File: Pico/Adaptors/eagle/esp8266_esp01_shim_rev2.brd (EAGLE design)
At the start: 15.9 x 11.9 mm, 4 parts, among them IC2 78L 3.3v

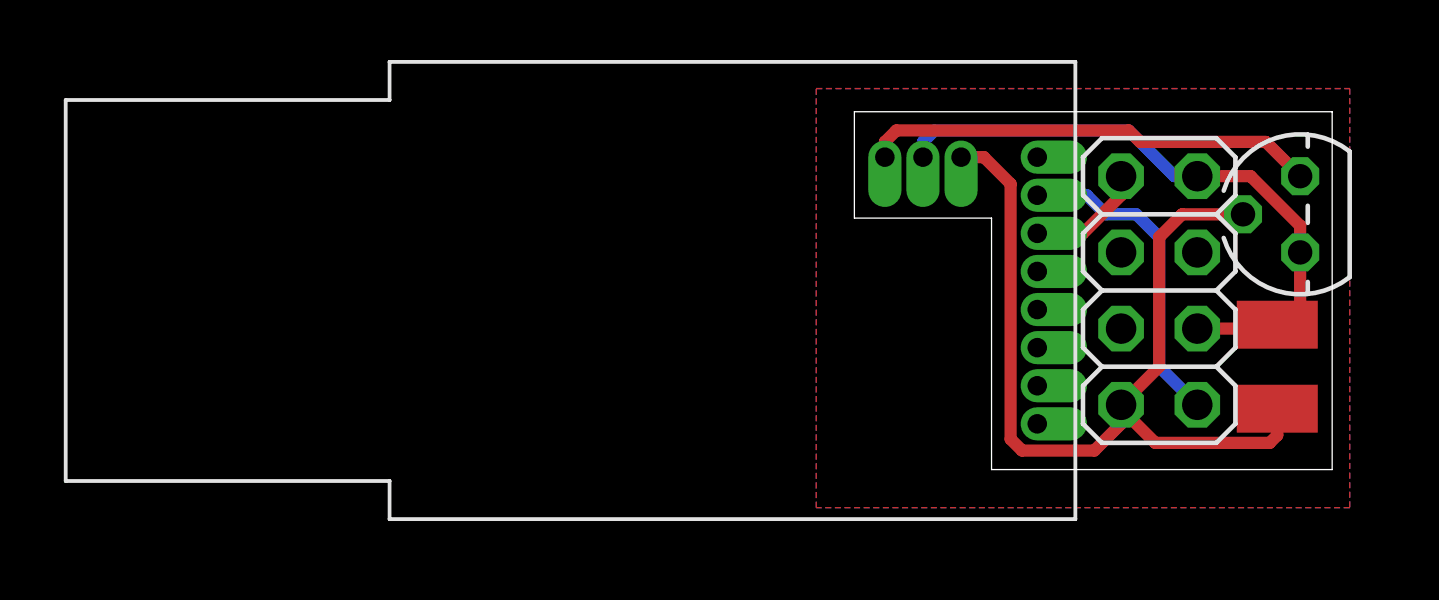
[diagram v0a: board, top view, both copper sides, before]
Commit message: tweak net classes
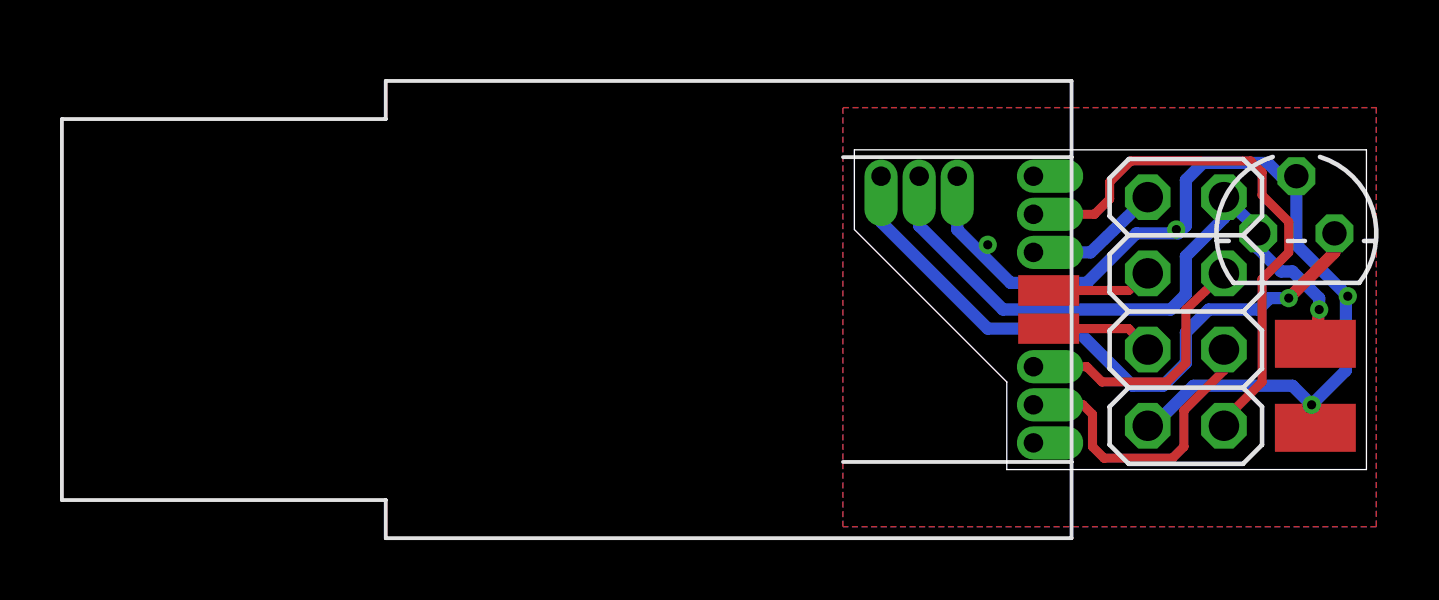
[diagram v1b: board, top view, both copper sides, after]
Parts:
- U$1: value ESPRUINO_PICO_0.05 -> ESPRUINO_PICO_0.05_SMALL; device espruino_pico:ESPRUINO_PICO_0.05 -> espruino_pico:ESPRUINO_PICO_0.05_SMALL
- moved C1 1.42 mm to (15.4, 2.79)
- moved U$1 1.31 mm to (0.89, 5.33)
- moved ESP8266 1.13 mm to (11.0, 5.27)
- moved IC2 0.65 mm to (14.7, 7.87), turned to 0 degrees
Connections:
- new net ESP_CH_PD: ESP8266.6, U$1.B9
- new net ESP_GPIO0: ESP8266.3, U$1.A1
- new net ESP_GPIO2: ESP8266.5, U$1.A0
- new net ESP_RST: ESP8266.4, U$1.A10
- net VCC: no longer ESP8266.6
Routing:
- net ESP_CH_PD: track 0.00 -> 10.3 mm
- net ESP_RST: track 0.00 -> 9.08 mm
- net ESP_TX: track 10.8 -> 18.6 mm
- net N$1: track 15.1 -> 22.0 mm, vias 0 -> 1
- net ESP_GPIO2: track 0.00 -> 3.61 mm
- net ESP_GPIO0: track 0.00 -> 3.52 mm
- net VCC: track 21.0 -> 22.6 mm, vias 0 -> 1
- net GND: track 31.4 -> 32.4 mm, vias 0 -> 4
- net ESP_RX: track 3.96 -> 4.55 mm
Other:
- board size 15.9 x 11.9 mm -> 17.1 x 10.7 mm
- board text added: "3.3"
- board text added: "47uF"
- board text added: "GND"
- board text added: "Vin"
